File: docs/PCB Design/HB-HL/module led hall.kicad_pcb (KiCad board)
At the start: 4 copper layers, 40 x 40 mm, 10 parts, among them J1 Conn_02x03_Top_Bottom, J2 Conn_01x04_MountingPin, U2 A3213LLHLT-T

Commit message: Directory rename and readme updated
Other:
- board text added: "HB-HL V.0.3"
- board text removed: "V.0.3"
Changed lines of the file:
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@@
 		(layer "Edge.Cuts")
 	)
-	(gr_text "V.0.3"
-		(at 80.75 103.25 -90)
+	(gr_text "HB-HL\nV.0.3"
+		(at 80.59 100.19 270)
 		(layer "B.SilkS")
 		(effects
@@
 				(bold yes)
 			)
-			(justify left bottom mirror)
+			(justify bottom mirror)
 		)
 	)
 	(gr_text "CIDCO.CA"
-		(at 82.95 105.7 -90)
+		(at 85.13 105.36 -90)
 		(layer "B.SilkS")
 		(effects

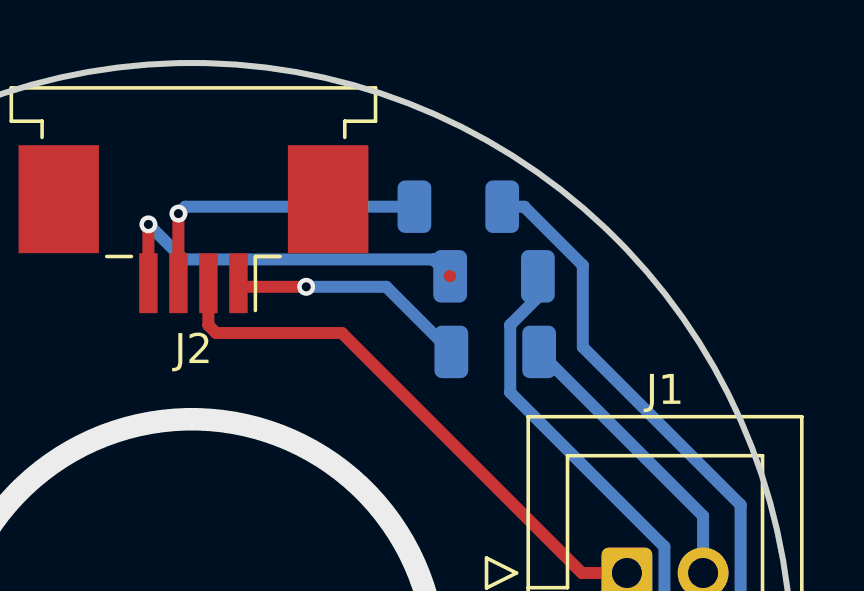
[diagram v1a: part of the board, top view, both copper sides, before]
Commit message: PCB Production files
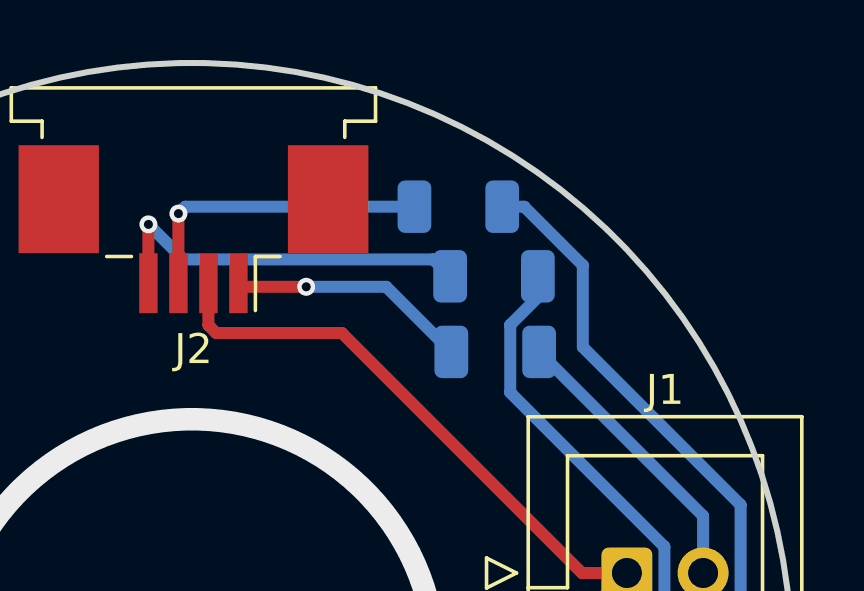
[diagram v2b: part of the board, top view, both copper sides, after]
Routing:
- net VCC: track 50.2 -> 48.8 mm
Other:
- copper layers 4 -> 2
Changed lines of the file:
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@@
 	(layers
 		(0 "F.Cu" signal)
-		(1 "In1.Cu" signal)
-		(2 "In2.Cu" signal)
 		(31 "B.Cu" signal)
 		(32 "B.Adhes" user "B.Adhesive")
@@
 			)
 			(layer "dielectric 1"
-				(type "prepreg")
-				(thickness 0.1)
-				(material "FR4")
-				(epsilon_r 4.5)
-				(loss_tangent 0.02)
-			)
-			(layer "In1.Cu"
-				(type "copper")
-				(thickness 0.035)
-			)
-			(layer "dielectric 2"
 				(type "core")
-				(thickness 1.24)
-				(material "FR4")
-				(epsilon_r 4.5)
-				(loss_tangent 0.02)
-			)
-			(layer "In2.Cu"
-				(type "copper")
-				(thickness 0.035)
-			)
-			(layer "dielectric 3"
-				(type "prepreg")
-				(thickness 0.1)
+				(thickness 1.51)
 				(material "FR4")
 				(epsilon_r 4.5)
@@
 		(property ki_fp_filters "Connector*:*_2x??_*")
 		(sheetname "Racine")
-		(sheetfile "module led et hall.kicad_sch")
+		(sheetfile "module led hall.kicad_sch")
 		(attr through_hole)
 		(fp_line
@@
 		(property ki_fp_filters "Connector*:*_1x??-1MP*")
 		(sheetname "Racine")
-		(sheetfile "module led et hall.kicad_sch")
+		(sheetfile "module led hall.kicad_sch")
 		(attr smd)
 		(fp_line
@@
 		(property ki_fp_filters "MountingHole*")
 		(sheetname "Racine")
-		(sheetfile "module led et hall.kicad_sch")
+		(sheetfile "module led hall.kicad_sch")
 		(attr exclude_from_pos_files exclude_from_bom)
 		(fp_circle
@@
 		(property ki_fp_filters "MountingHole*")
 		(sheetname "Racine")
-		(sheetfile "module led et hall.kicad_sch")
+		(sheetfile "module led hall.kicad_sch")
 		(attr exclude_from_pos_files exclude_from_bom)
 		(fp_circle
@@
 		(property ki_fp_filters "R_*")
 		(sheetname "Racine")
-		(sheetfile "module led et hall.kicad_sch")
+		(sheetfile "module led hall.kicad_sch")
 		(attr smd)
 		(fp_line
@@
 		(property ki_fp_filters "C_*")
 		(sheetname "Racine")
-		(sheetfile "module led et hall.kicad_sch")
+		(sheetfile "module led hall.kicad_sch")
 		(attr smd)
 		(fp_line
@@
 		(property ki_fp_filters "R_*")
 		(sheetname "Racine")
-		(sheetfile "module led et hall.kicad_sch")
+		(sheetfile "module led hall.kicad_sch")
 		(attr smd)
 		(fp_line
@@
 		(property ki_fp_filters "R_*")
 		(sheetname "Racine")
-		(sheetfile "module led et hall.kicad_sch")
+		(sheetfile "module led hall.kicad_sch")
 		(attr smd)
 		(fp_line
@@
 		(property ki_fp_filters "SOT?23W*")
 		(sheetname "Racine")
-		(sheetfile "module led et hall.kicad_sch")
+		(sheetfile "module led hall.kicad_sch")
 		(attr smd)
 		(fp_line
@@
 		(property ki_fp_filters "C_*")
 		(sheetname "Racine")
-		(sheetfile "module led et hall.kicad_sch")
+		(sheetfile "module led hall.kicad_sch")
 		(attr smd)
 		(fp_line
@@
 	(segment
 		(start 114.5 97)
-		(end 113.122035 97)
-		(width 0.4)
-		(layer "In1.Cu")
-		(net 1)
-	)
-	(segment
-		(start 114.5 97)
 		(end 112.36 99.14)
 		(width 0.4)
@@
 	)
 	(segment
-		(start 108.5975 87.1)
-		(end 108.6075 87.11)
-		(width 0.4)
-		(layer "F.Cu")
-		(net 9)
-	)
-	(segment
